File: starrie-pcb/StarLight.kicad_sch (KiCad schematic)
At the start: 18 parts, among them J1 Conn_01x02_Socket, U1 NE555P, U2 4017

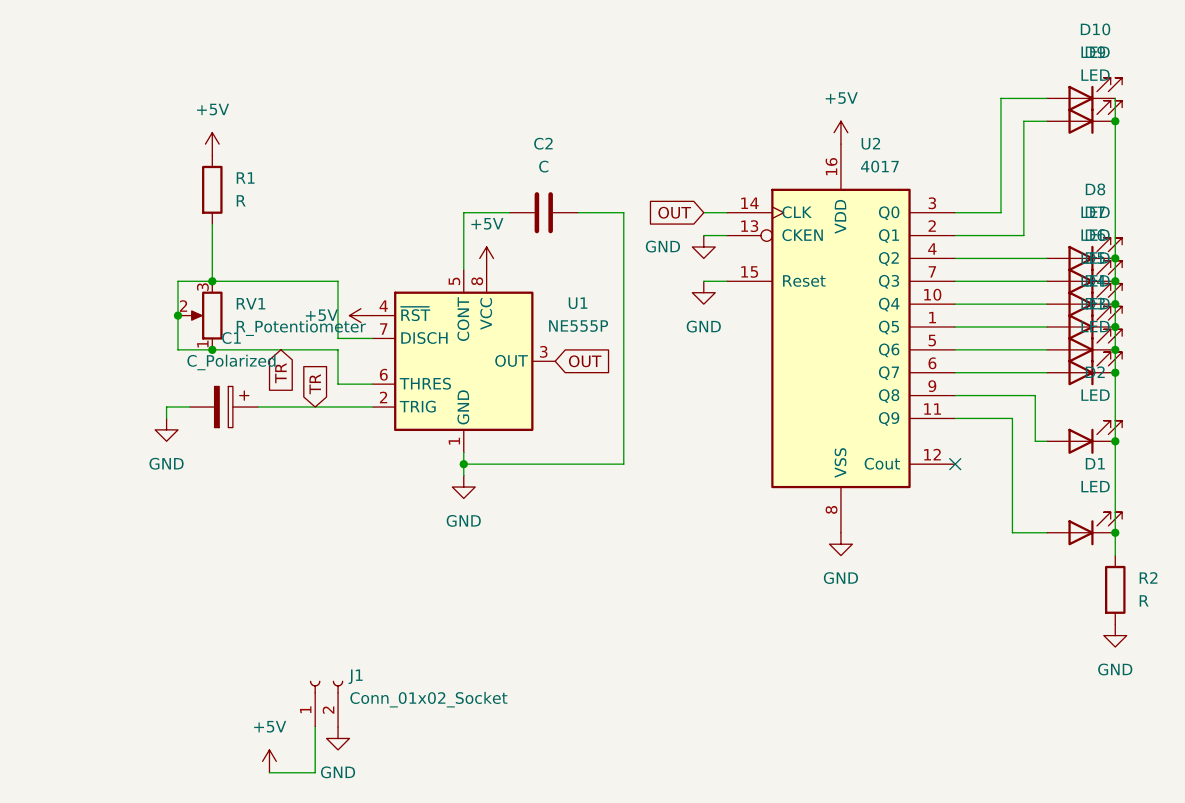
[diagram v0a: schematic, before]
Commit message: NEW GERBERS
this better be right or im gonna lose it. this is my last time ordering the pcb if it fails this time too i will do unspeakable things
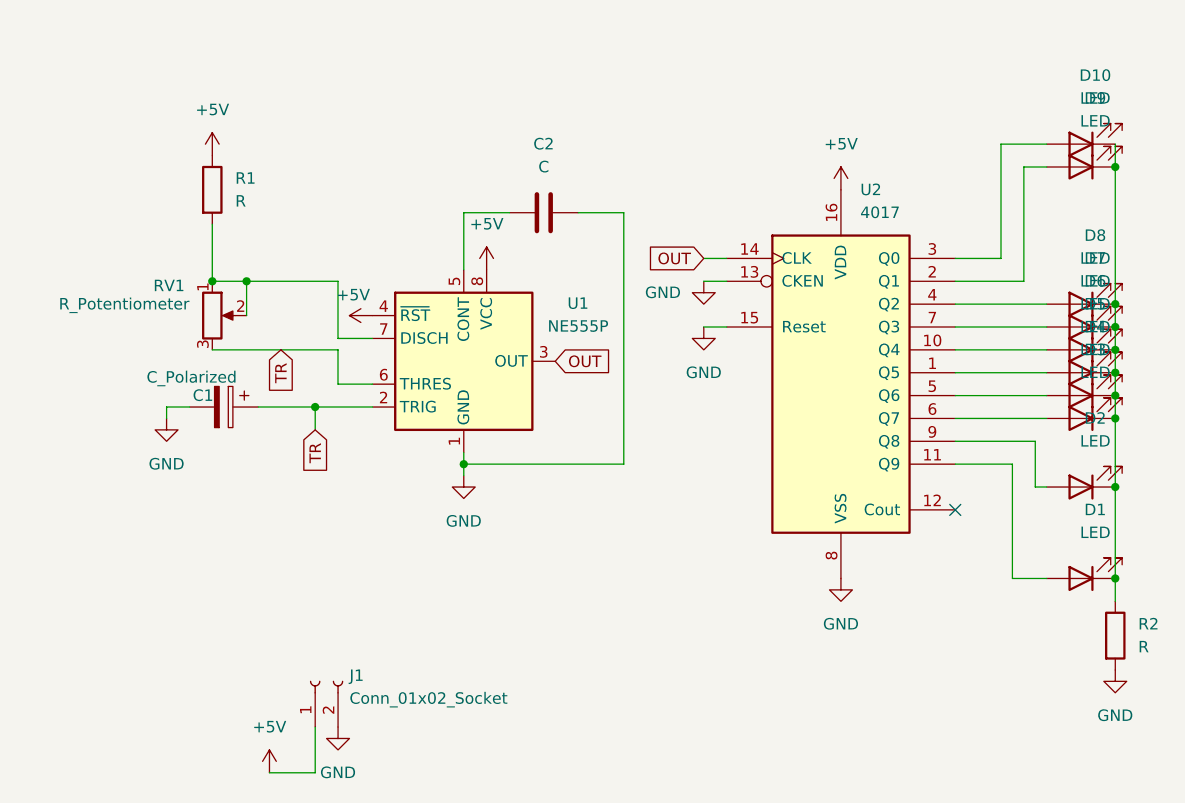
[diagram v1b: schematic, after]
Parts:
- U2: footprint footprints1:N16 -> cd4017:N16
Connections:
- net TR: no longer R1.2, RV1.1, RV1.2, U1.7 (DISCH)
- new net: R1.2, RV1.1, RV1.2, U1.7 (DISCH)
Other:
- moved on the sheet: D1, D10, D2, D3, D4, D5, D6, D7, D8, D9, R2, RV1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
